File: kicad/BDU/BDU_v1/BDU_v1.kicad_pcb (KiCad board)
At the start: 2 copper layers, 140 x 60 mm, 44 parts, among them J1 Relay connector, J10 Voltmeter-, J11 IMD-, J12 AIR-, J13 AIR+, J16 DCDC, J17 AMS, J2 Relay connector, J3 Relay connector, J4 Conn_01x02, J5 IMD+, J6 Voltmeter+, J7 TSAL_green+, J8 AIR+, J9 TSAL_green-, U1 LTV-847S, U2 TRA3-1212

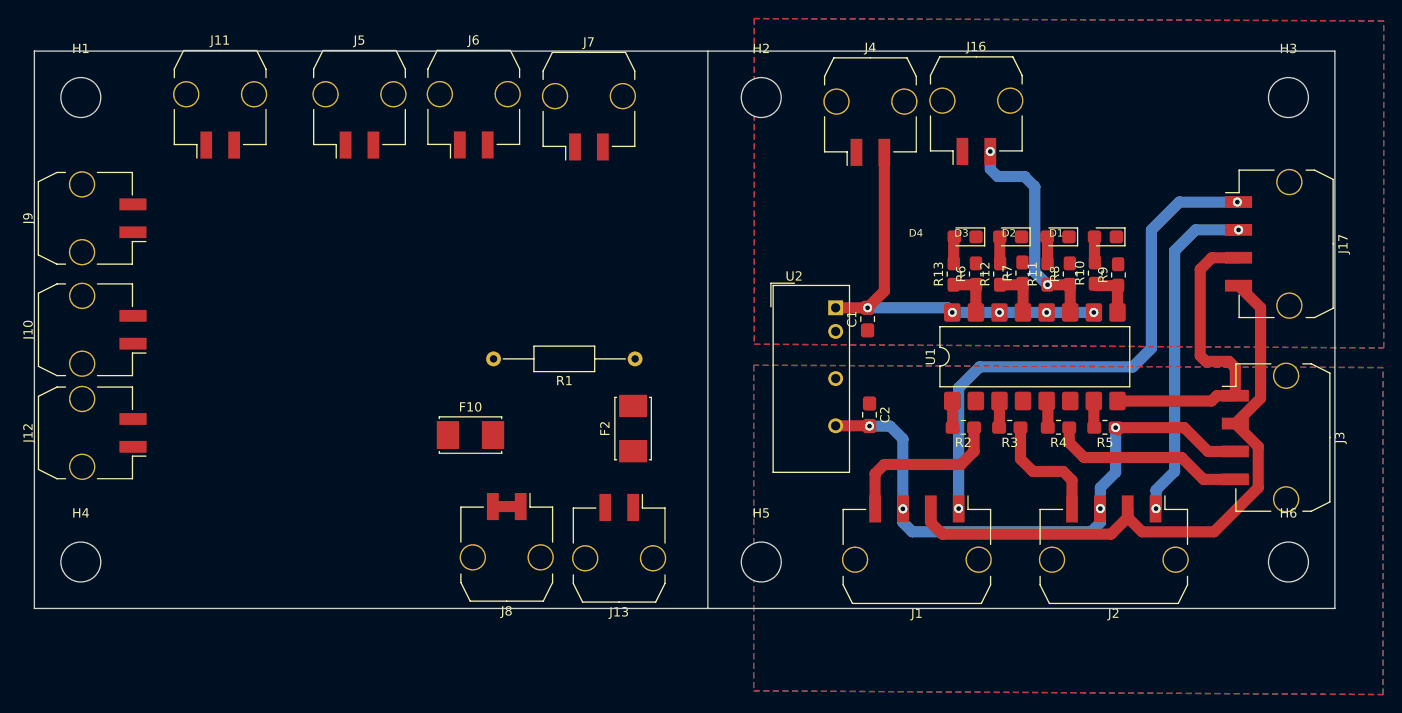
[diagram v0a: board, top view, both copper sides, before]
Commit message: SSRU new layout
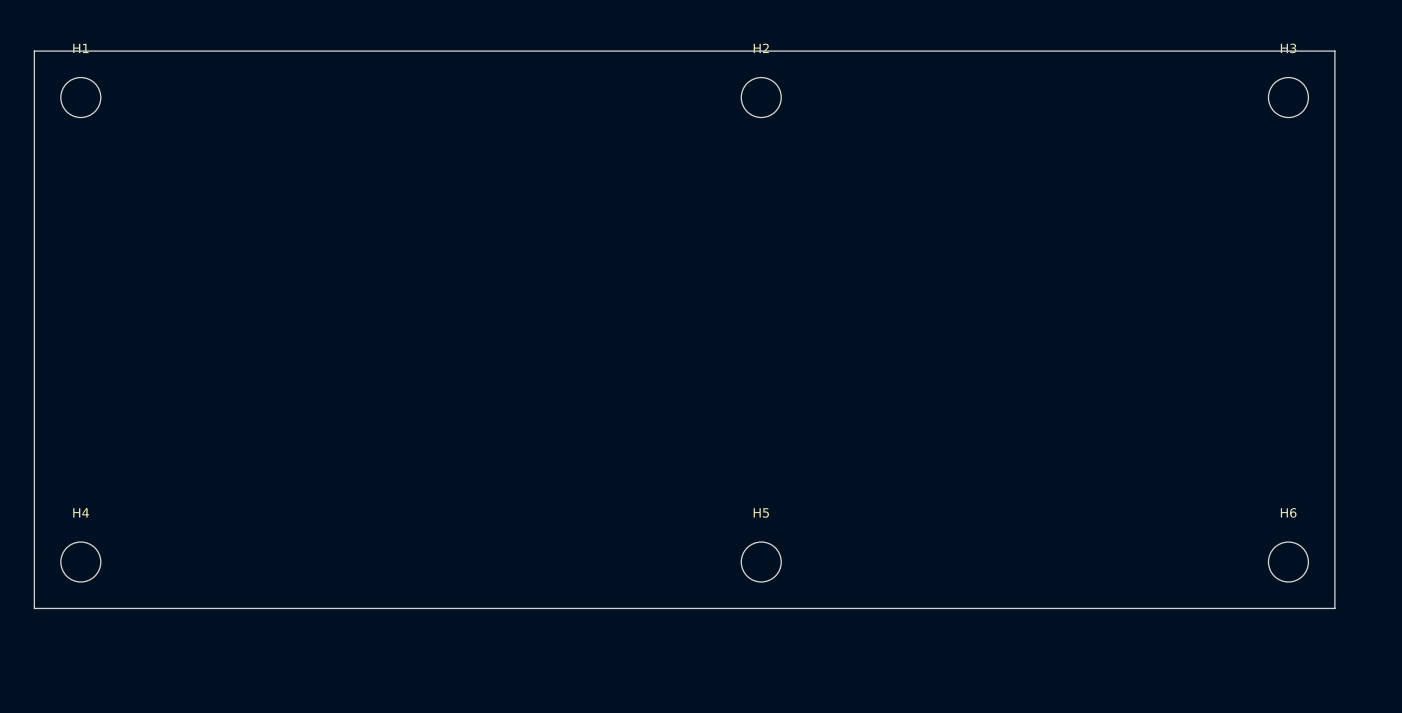
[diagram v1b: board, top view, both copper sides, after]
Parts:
- removed C1: 2.2uF, RMC_Capacitor:C_0805_2012Metric_Pad1.18x1.45mm_HandSolder_L
- removed C2: 1uF, RMC_Capacitor:C_0805_2012Metric_Pad1.18x1.45mm_HandSolder_L
- removed D1, D2, D3, D4: LED, RMC_LED:LED_0805_2012Metric_Pad1.45x1.40mm_HandSolder
- removed F10, F2: Fuse, Fuse:Fuseholder_Littelfuse_Nano2_157x
- removed J1, J2, J3: Relay connector, Connector_Molex:Molex_Micro-Fit_3.0_43650-0410_1x04-1MP_P3.00mm_Horizontal_PnP
- removed J10: Voltmeter-, Connector_Molex:Molex_Micro-Fit_3.0_43650-0210_1x02-1MP_P3.00mm_Horizontal_PnP
- removed J11: IMD-, Connector_Molex:Molex_Micro-Fit_3.0_43650-0210_1x02-1MP_P3.00mm_Horizontal_PnP
- removed J12: AIR-, Connector_Molex:Molex_Micro-Fit_3.0_43650-0210_1x02-1MP_P3.00mm_Horizontal_PnP
- removed J13, J8: AIR+, Connector_Molex:Molex_Micro-Fit_3.0_43650-0210_1x02-1MP_P3.00mm_Horizontal_PnP
- removed J16: DCDC, Connector_Molex:Molex_Micro-Fit_3.0_43650-0210_1x02-1MP_P3.00mm_Horizontal_PnP
- removed J17: AMS, Connector_Molex:Molex_Micro-Fit_3.0_43650-0410_1x04-1MP_P3.00mm_Horizontal_PnP
- removed J4: Conn_01x02, Connector_Molex:Molex_Micro-Fit_3.0_43650-0210_1x02-1MP_P3.00mm_Horizontal_PnP
- removed J5: IMD+, Connector_Molex:Molex_Micro-Fit_3.0_43650-0210_1x02-1MP_P3.00mm_Horizontal_PnP
- removed J6: Voltmeter+, Connector_Molex:Molex_Micro-Fit_3.0_43650-0210_1x02-1MP_P3.00mm_Horizontal_PnP
- removed J7: TSAL_green+, Connector_Molex:Molex_Micro-Fit_3.0_43650-0210_1x02-1MP_P3.00mm_Horizontal_PnP
- removed J9: TSAL_green-, Connector_Molex:Molex_Micro-Fit_3.0_43650-0210_1x02-1MP_P3.00mm_Horizontal_PnP
- removed R1: 3K9, Resistor_THT:R_Axial_DIN0207_L6.3mm_D2.5mm_P15.24mm_Horizontal
- removed R10, R11, R12, R13, R2, R3, R4, R5: 1k, RMC_Resistor:R_0805_2012Metric_Pad1.20x1.40mm_HandSolder_L
- removed R6, R7, R8, R9: 4k7, RMC_Resistor:R_0805_2012Metric_Pad1.20x1.40mm_HandSolder_L
- removed U1: LTV-847S, Package_DIP:SMDIP-16_W9.53mm
- removed U2: TRA3-1212, Converter_DCDC:Converter_DCDC_TRACO_TRA3-xxxx_THT
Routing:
- net SDC+: track 66.4 -> 0.00 mm
- net +12VA: track 64.2 -> 0.00 mm, vias 4 -> 0
- net AIR_H-: track 58.9 -> 0.00 mm, vias 2 -> 0
- net +12V: track 45.5 -> 0.00 mm, vias 5 -> 0
- net AIR_L-: track 36.5 -> 0.00 mm, vias 2 -> 0
- net PRE-: track 34.2 -> 0.00 mm
- net /pre_out: track 24.0 -> 0.00 mm, vias 2 -> 0
- net /pre_aux: track 21.1 -> 0.00 mm
- net /high_aux: track 18.0 -> 0.00 mm
- net /low_aux: track 12.9 -> 0.00 mm
- net /low_out: track 5.55 -> 0.00 mm
- net /sdc_out: track 5.50 -> 0.00 mm
- net /high_out: track 5.39 -> 0.00 mm
- net TS+: track 3.00 -> 0.00 mm
- net Net-(R4-Pad2): track 2.92 -> 0.00 mm
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- removed copper zone on B.Cu, net GND
- removed copper zone on F.Cu, net GND
- removed copper zone on B.Cu, net GNDA
- removed copper zone on F.Cu, net GNDA
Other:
- outline, holes or cut-outs redrawn
